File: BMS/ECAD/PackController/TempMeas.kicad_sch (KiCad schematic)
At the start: 2 parts

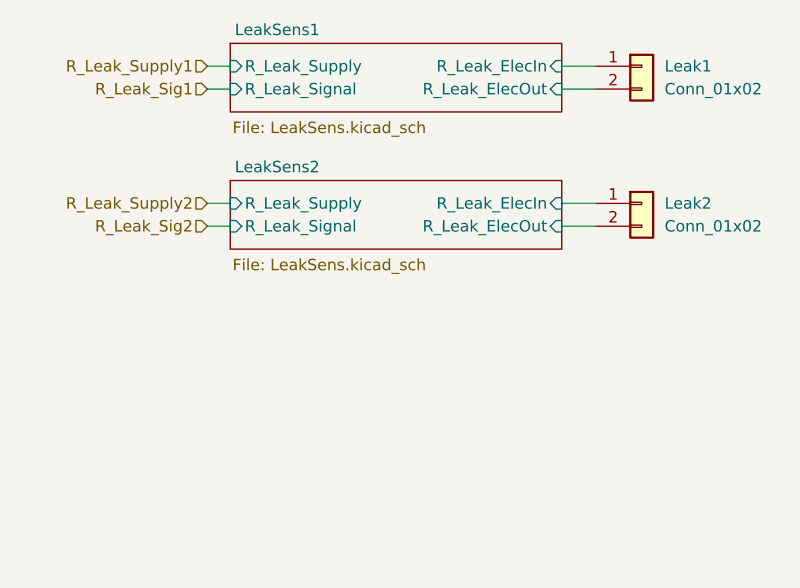
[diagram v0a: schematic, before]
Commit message: schematic finished, review tbd
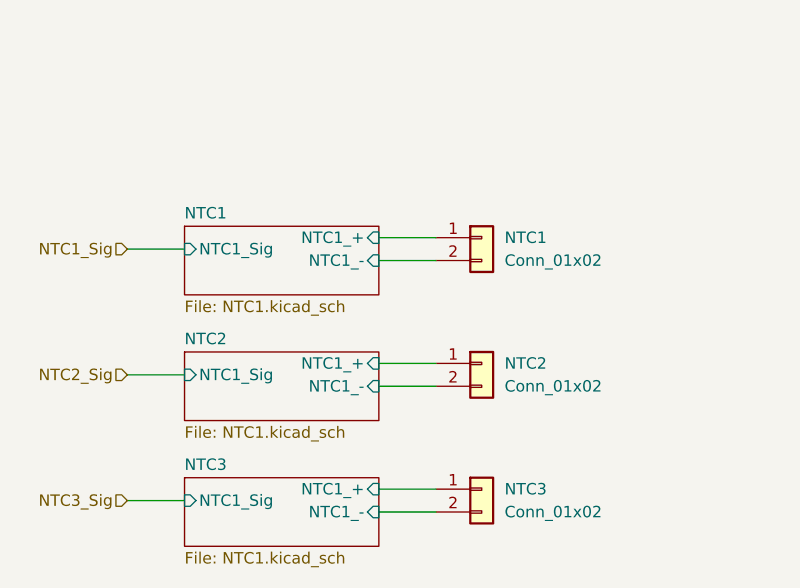
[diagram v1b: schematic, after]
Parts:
- removed Leak1, Leak2: Conn_01x02, symbol Connector_Generic:Conn_01x02
- added NTC1, NTC2, NTC3: Conn_01x02, symbol Connector_Generic:Conn_01x02
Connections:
- new net NTC1/NTC1_+: NTC1.1 (Pin_1)
- new net NTC1/NTC1_-: NTC1.2 (Pin_2)
- new net NTC2/NTC1_+: NTC2.1 (Pin_1)
- new net NTC2/NTC1_-: NTC2.2 (Pin_2)
- new net NTC3/NTC1_+: NTC3.1 (Pin_1)
- new net NTC3/NTC1_-: NTC3.2 (Pin_2)
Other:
- removed sheet LeakSens1
- removed sheet LeakSens2
- added sheet NTC1 (NTC1.kicad_sch)
- added sheet NTC2 (NTC1.kicad_sch)
- added sheet NTC3 (NTC1.kicad_sch)
